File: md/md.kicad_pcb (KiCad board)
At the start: 2 copper layers, 59.7 x 67.3 mm, 55 parts, among them J1 OutB, J2 OutA, J3 Interface, J4 12VJmp, J5 Conn_02x08_Counter_Clockwise, J6 Conn_02x08_Counter_Clockwise, J7 Conn_02x08_Counter_Clockwise, J8 Conn_02x08_Counter_Clockwise, Q1 FETA(IRFB7437PBF), Q2 FETA(IRFB7437PBF), Q3 FETB(IRFB7437PBF), Q4 FETB(IRFB7437PBF), U1 TLP2105, U2 IR7184S, U3 IR7184S, U4 7400, U5 L7812

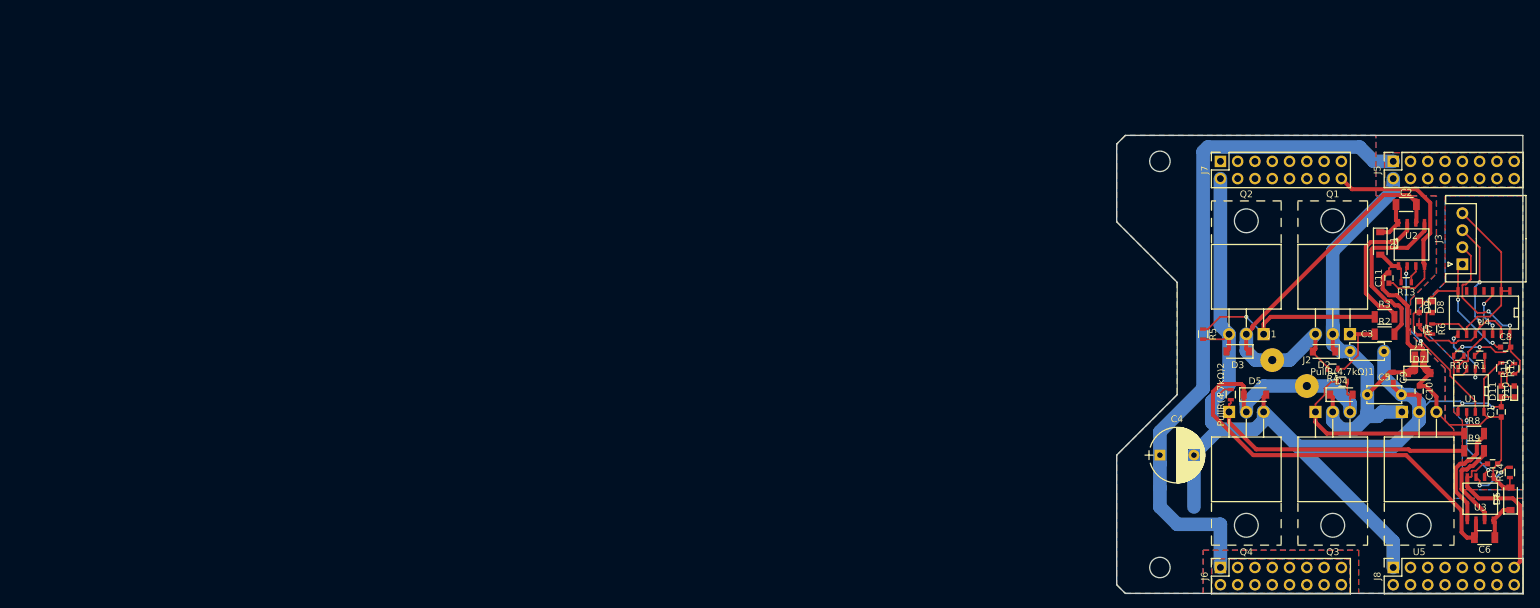
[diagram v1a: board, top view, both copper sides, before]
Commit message: update pcb
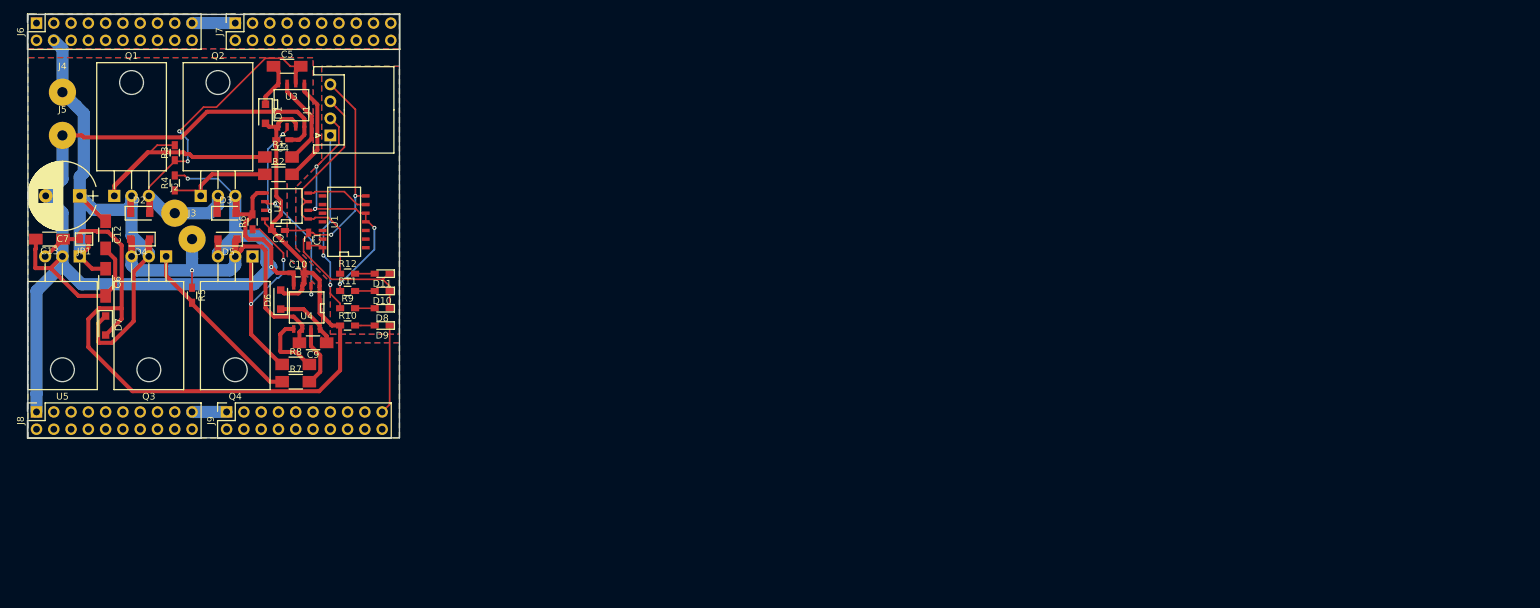
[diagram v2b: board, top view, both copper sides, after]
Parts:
- removed C11, C8: C, Capacitors_SMD:C_0603
- removed C3: PowerC, Capacitors_THT:C_Disc_D5.0mm_W2.5mm_P5.00mm
- removed PullR(4.7kΩ)1, PullR(4.7kΩ)2: R, Resistors_SMD:R_0603
- removed R13, R14: PullR, Resistors_SMD:R_0603
- added C12: 10uF, Capacitors_SMD:C_1206_HandSoldering, F.Cu at (24.1, 71.8)
- added C13: 10uF, Capacitors_SMD:C_1206_HandSoldering, F.Cu at (15.9, 72.4)
- added J9: PWR_INPUT+, Socket_Strips:Socket_Strip_Straight_2x10_Pitch2.54mm, F.Cu at (41.9, 97.8)
- added JP1: USE_12V, Connectors:GS2, F.Cu at (21.0, 72.4)
- C1: footprint Capacitors_SMD:C_0603 -> Capacitors_SMD:C_0603_HandSoldering
- C10: value RegOutC(1uF) -> 0.1uF; footprint Capacitors_SMD:C_0603 -> Capacitors_SMD:C_0603_HandSoldering
- C2: value BootC(10uF) -> 0.1uF; footprint Capacitors_SMD:C_1206 -> Capacitors_SMD:C_0603_HandSoldering
- C4: value PowerCP -> 0.1uF; footprint Capacitors_THT:CP_Radial_D8.0mm_P5.00mm -> Capacitors_SMD:C_0603_HandSoldering
- C5: value PowerC -> 10uF; footprint Capacitors_THT:C_Disc_D5.0mm_W2.5mm_P5.00mm -> Capacitors_SMD:C_1206_HandSoldering
- C6: value BootC(10uF) -> 10uF; footprint Capacitors_SMD:C_1206 -> Capacitors_SMD:C_1206_HandSoldering
- C7: value 0.1uF -> 470uF; footprint Capacitors_SMD:C_0603 -> Capacitors_THT:CP_Radial_D10.0mm_P5.00mm
- C9: value RegInC(1uF) -> 10uF; footprint Capacitors_SMD:C_0603 -> Capacitors_SMD:C_1206_HandSoldering
- D1, D6: footprint Diodes_SMD:D_SOD-123 -> Diodes_SMD:D_SOD-123F
- D10: value 5VLED(SML-E12P8T86) -> OSYL; footprint LEDs:LED_0603 -> LEDs:LED_0603_HandSoldering
- D11: value 12VLED(SML-E12V8WT86) -> OSHR; footprint LEDs:LED_0603 -> LEDs:LED_0603_HandSoldering
- D2, D3, D4, D5: value RevD(SS2040FL) -> SS2040FL; footprint Diodes_SMD:D_SOD-123 -> Diodes_SMD:D_SOD-123F
- D7: value RegRevC(SS2040FL) -> SS2040FL; footprint Diodes_SMD:D_SOD-123 -> Diodes_SMD:D_SOD-123F
- D8: value DIRLED(SML-E12Y8WT86) -> OSBL; footprint LEDs:LED_0603 -> LEDs:LED_0603_HandSoldering
- D9: value LED(SML-E13BC8TT86) -> OSWT; footprint LEDs:LED_0603 -> LEDs:LED_0603_HandSoldering
- J1: value OutB -> CONTROLL; footprint Wire_Pads:SolderWirePad_single_1-2mmDrill -> Connectors_JST:JST_XH_S04B-XH-A_04x2.50mm_Angled
- J2: value OutA -> OUTA; footprint Wire_Pads:SolderWirePad_single_1-2mmDrill -> Wire_Pads:SolderWirePad_single_1-5mmDrill
- J3: value Interface -> OUTB; footprint Connectors_JST:JST_XH_S04B-XH-A_04x2.50mm_Angled -> Wire_Pads:SolderWirePad_single_1-5mmDrill
- J4: value 12VJmp -> PWR_INPUT+; footprint Connectors:GS2 -> Wire_Pads:SolderWirePad_single_1-5mmDrill
- J5: value Conn_02x08_Counter_Clockwise -> PWR_INPUT-; footprint Socket_Strips:Socket_Strip_Straight_2x08_Pitch2.54mm -> Wire_Pads:SolderWirePad_single_1-5mmDrill
- J6, J7, J8: value Conn_02x08_Counter_Clockwise -> PWR_INPUT+; footprint Socket_Strips:Socket_Strip_Straight_2x08_Pitch2.54mm -> Socket_Strips:Socket_Strip_Straight_2x10_Pitch2.54mm
- Q1, Q2: value FETA(IRFB7437PBF) -> IRFB7437PBF; footprint TO_SOT_Packages_THT:TO-220-3_Horizontal_Reversed -> TO_SOT_Packages_THT:TO-220-3_Horizontal
- Q3, Q4: value FETB(IRFB7437PBF) -> IRFB7437PBF; footprint TO_SOT_Packages_THT:TO-220-3_Horizontal_Reversed -> TO_SOT_Packages_THT:TO-220-3_Horizontal
- R1: value TLP_R(470Ω) -> 10Ω; footprint Resistors_SMD:R_0603 -> Resistors_SMD:R_1206_HandSoldering
- R10: value TLP_R(470Ω) -> 470Ω; footprint Resistors_SMD:R_0603 -> Resistors_SMD:R_0603_HandSoldering
- R11: value 5VLEDR(470Ω) -> 220Ω; footprint Resistors_SMD:R_0603 -> Resistors_SMD:R_0603_HandSoldering
- R12: value 12VLEDR(1.2kΩ) -> 220Ω; footprint Resistors_SMD:R_0603 -> Resistors_SMD:R_0603_HandSoldering
- R2, R8: value GateR(8.2Ω) -> 10Ω; footprint Resistors_SMD:R_1206 -> Resistors_SMD:R_1206_HandSoldering
- R3: value GateR(8.2Ω) -> 4.7kΩ; footprint Resistors_SMD:R_1206 -> Resistors_SMD:R_0603_HandSoldering
- R4, R5: value PullR(4.7kΩ) -> 4.7kΩ; footprint Resistors_SMD:R_0603 -> Resistors_SMD:R_0603_HandSoldering
- R6: value DIRLEDR(470Ω) -> 4.7kΩ; footprint Resistors_SMD:R_0603 -> Resistors_SMD:R_0603_HandSoldering
- R7: value PWMLEDR(470Ω) -> 10Ω; footprint Resistors_SMD:R_0603 -> Resistors_SMD:R_1206_HandSoldering
- R9: value GateR(8.2Ω) -> 150Ω; footprint Resistors_SMD:R_1206 -> Resistors_SMD:R_0603_HandSoldering
- U1: value TLP2105 -> 74HC00; footprint SMD_Packages:SOIC-8-N -> SMD_Packages:SOIC-14_N
- U2: value IR7184S -> TLP2105
- U4: value 7400 -> IR7184S; footprint SMD_Packages:SOIC-14_N -> SMD_Packages:SOIC-8-N
- U5: value L7812 -> LM7812_TO220; footprint TO_SOT_Packages_THT:TO-220-3_Horizontal_Reversed -> TO_SOT_Packages_THT:TO-220-3_Horizontal
- moved C7 211.3 mm to (20.3, 66.0)
- moved C6 206.1 mm to (24.1, 78.7), turned to 270 degrees
- moved J4 203.1 mm to (17.8, 50.8), turned to 0 degrees
- moved J8 200.7 mm to (14.0, 97.8)
- moved U5 195.7 mm to (20.3, 74.9), turned to 180 degrees
- moved J5 195.6 mm to (17.8, 57.1), turned to 0 degrees
- moved D7 193.2 mm to (24.1, 85.1), turned to 270 degrees
- moved J6 191.5 mm to (14.0, 40.6)
- moved J3 186.7 mm to (36.8, 72.4), turned to 0 degrees
- moved U3 184.0 mm to (51.4, 52.7), turned to 0 degrees
- moved D6 183.1 mm to (49.9, 81.3)
- moved Q1 182.7 mm to (25.4, 66.0), turned to 0 degrees
- moved R3 179.4 mm to (34.3, 59.7), turned to 90 degrees
- moved R1 178.9 mm to (49.5, 60.3), turned to 0 degrees
- moved D4 178.0 mm to (29.2, 72.4), turned to 180 degrees
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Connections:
- C1 pad 1: +12V -> GND
- C1 pad 2: GNDPWR -> +5V
- C10 pad 1: +12V -> GNDPWR
- C10 pad 2: GNDPWR -> +12V
- C2 pad 1: Net-(C2-Pad1) -> GND
- C2 pad 2: Net-(C2-Pad2) -> +12V
- C4 pad 1: +24V -> GNDPWR
- C4 pad 2: GNDPWR -> +12V
- C5 pad 1: +24V -> Net-(C5-Pad1)
- C5 pad 2: GNDPWR -> Net-(C5-Pad2)
- C6 pad 1: Net-(C6-Pad1) -> +24V
- C6 pad 2: Net-(C6-Pad2) -> GNDPWR
- C7 pad 1: +12V -> +24V
- C9 pad 1: +24V -> Net-(C9-Pad1)
- C9 pad 2: GNDPWR -> Net-(C9-Pad2)
- D1 pad 1: Net-(C2-Pad1) -> Net-(C5-Pad1)
- D10 pad 1: GNDPWR -> GND
- D11 pad 1: GNDPWR -> GND
- D2 pad 2: Net-(C2-Pad2) -> Net-(C5-Pad2)
- D3 pad 1: Net-(C2-Pad2) -> Net-(C5-Pad2)
- D4 pad 2: Net-(C6-Pad2) -> Net-(C9-Pad2)
- D5 pad 1: Net-(C6-Pad2) -> Net-(C9-Pad2)
- D6 pad 1: Net-(C6-Pad1) -> Net-(C9-Pad1)
- D9 pad 1: GND -> GNDPWR
- J1 pad 1: Net-(C2-Pad2) -> +5V
- J2 pad 1: Net-(C6-Pad2) -> Net-(C5-Pad2)
- J3 pad 1: GND -> Net-(C9-Pad2)
- J5 pad 1: +24V -> GNDPWR
- J7 pad 1: GNDPWR -> +24V
- J7 pad 10: GNDPWR -> +24V
- J7 pad 11: GNDPWR -> +24V
- J7 pad 12: GNDPWR -> +24V
- J7 pad 13: GNDPWR -> +24V
- J7 pad 14: GNDPWR -> +24V
- J7 pad 15: GNDPWR -> +24V
- J7 pad 16: GNDPWR -> +24V
- J7 pad 2: GNDPWR -> +24V
- J7 pad 3: GNDPWR -> +24V
- J7 pad 4: GNDPWR -> +24V
- J7 pad 5: GNDPWR -> +24V
- J7 pad 6: GNDPWR -> +24V
- J7 pad 7: GNDPWR -> +24V
- J7 pad 8: GNDPWR -> +24V
- J7 pad 9: GNDPWR -> +24V
- Q1 pad 3: Net-(C2-Pad2) -> Net-(C5-Pad2)
- Q2 pad 2: Net-(C2-Pad2) -> Net-(C5-Pad2)
- Q3 pad 1: Net-(PullR(4.7kΩ)1-Pad1) -> Net-(Q3-Pad1)
- Q3 pad 3: Net-(C6-Pad2) -> Net-(C9-Pad2)
- Q4 pad 1: Net-(PullR(4.7kΩ)2-Pad1) -> Net-(Q4-Pad1)
- Q4 pad 2: Net-(C6-Pad2) -> Net-(C9-Pad2)
- R1 pad 1: Net-(R1-Pad1) -> Net-(Q1-Pad1)
- R1 pad 2: +5V -> Net-(R1-Pad2)
- R10 pad 1: Net-(R10-Pad1) -> +12V
- R10 pad 2: +5V -> Net-(D9-Pad2)
- R11 pad 1: +5V -> /DIR
- R12 pad 1: +12V -> /PWM
- R2 pad 1: Net-(Q1-Pad1) -> Net-(Q2-Pad1)
- R3 pad 1: Net-(Q2-Pad1) -> Net-(C5-Pad2)
- R3 pad 2: Net-(R3-Pad2) -> Net-(Q1-Pad1)
- R4 pad 1: Net-(Q1-Pad1) -> Net-(Q2-Pad1)
- R4 pad 2: Net-(C2-Pad2) -> GNDPWR
- R5 pad 1: Net-(Q2-Pad1) -> Net-(C9-Pad2)
- R5 pad 2: GNDPWR -> Net-(Q3-Pad1)
- R6 pad 1: /DIR -> Net-(Q4-Pad1)
- R6 pad 2: Net-(D8-Pad2) -> GNDPWR
- R7 pad 1: /PWM -> Net-(Q3-Pad1)
- R7 pad 2: Net-(D9-Pad2) -> Net-(R7-Pad2)
- R8 pad 1: Net-(PullR(4.7kΩ)1-Pad1) -> Net-(Q4-Pad1)
- R9 pad 1: Net-(PullR(4.7kΩ)2-Pad1) -> +5V
- R9 pad 2: Net-(R9-Pad2) -> Net-(D8-Pad2)
- U1 pad 1: Net-(R1-Pad1) -> (no net)
- U1 pad 2: Net-(U1-Pad2) -> (no net)
- U1 pad 3: Net-(R10-Pad1) -> (no net)
- U1 pad 4: Net-(U1-Pad4) -> /DIR
- U1 pad 5: GNDPWR -> /DIR
- U1 pad 6: /OUTB -> Net-(U1-Pad6)
- U1 pad 7: /OUTA -> GND
- U1 pad 8: +12V -> (no net)
- U2 pad 1: +12V -> /PWM
- U2 pad 2: /OUTA -> /DIR
- U2 pad 3: Net-(R13-Pad1) -> /PWM
- U2 pad 4: GNDPWR -> Net-(U1-Pad6)
- U2 pad 5: Net-(R2-Pad2) -> GNDPWR
- U2 pad 6: Net-(C2-Pad2) -> /OUTB
- U2 pad 7: Net-(R3-Pad2) -> /OUTA
- U2 pad 8: Net-(C2-Pad1) -> +12V
- U3 pad 2: /OUTB -> /OUTA
- U3 pad 3: Net-(R14-Pad2) -> +12V
- U3 pad 5: Net-(R8-Pad2) -> Net-(R2-Pad2)
- U3 pad 6: Net-(C6-Pad2) -> Net-(C5-Pad2)
- U3 pad 7: Net-(R9-Pad2) -> Net-(R1-Pad2)
- U3 pad 8: Net-(C6-Pad1) -> Net-(C5-Pad1)
- U4 pad 1: /DIR -> +12V
- U4 pad 2: /DIR -> /OUTB
- U4 pad 3: Net-(U4-Pad12) -> +12V
- U4 pad 4: Net-(U4-Pad4) -> GNDPWR
- U4 pad 5: Net-(U4-Pad5) -> Net-(R8-Pad2)
- U4 pad 6: Net-(U4-Pad6) -> Net-(C9-Pad2)
- U4 pad 7: GND -> Net-(R7-Pad2)
- U4 pad 8: Net-(U1-Pad2) -> Net-(C9-Pad1)
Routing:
- net Net-(C6-Pad2): track 88.0 -> 0.00 mm
- net +24V: track 174.3 -> 99.6 mm
- net +12V: track 72.9 -> 141.1 mm
- net Net-(C2-Pad2): track 60.8 -> 0.00 mm
- net Net-(C5-Pad2): track 0.00 -> 57.6 mm, vias 0 -> 2
- net Net-(C9-Pad2): track 0.00 -> 54.0 mm, vias 0 -> 1
- net Net-(PullR(4.7kΩ)2-Pad1): track 39.8 -> 0.00 mm
- net GND: track 22.3 -> 56.1 mm
- net Net-(Q4-Pad1): track 0.00 -> 33.5 mm, vias 0 -> 2
- net Net-(PullR(4.7kΩ)1-Pad1): track 30.3 -> 0.00 mm
- net Net-(Q1-Pad1): track 11.7 -> 38.6 mm
- net Net-(Q3-Pad1): track 0.00 -> 26.5 mm
- net Net-(R3-Pad2): track 20.9 -> 0.00 mm
- net Net-(R9-Pad2): track 13.6 -> 0.00 mm
- net Net-(R1-Pad2): track 0.00 -> 13.6 mm
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- added copper zone on B.Cu, net +12V
- removed copper zone on B.Cu, net +24V
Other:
- board size 59.7 x 67.3 mm -> 54.6 x 62.2 mm
